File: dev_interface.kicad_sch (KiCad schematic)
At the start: 17 parts, among them U10 ADS1014IDGS, U11 ADS1014IDGS, U4 ISO164xB, U5 DACx53401, U6 DACx53401, U8 LM2904

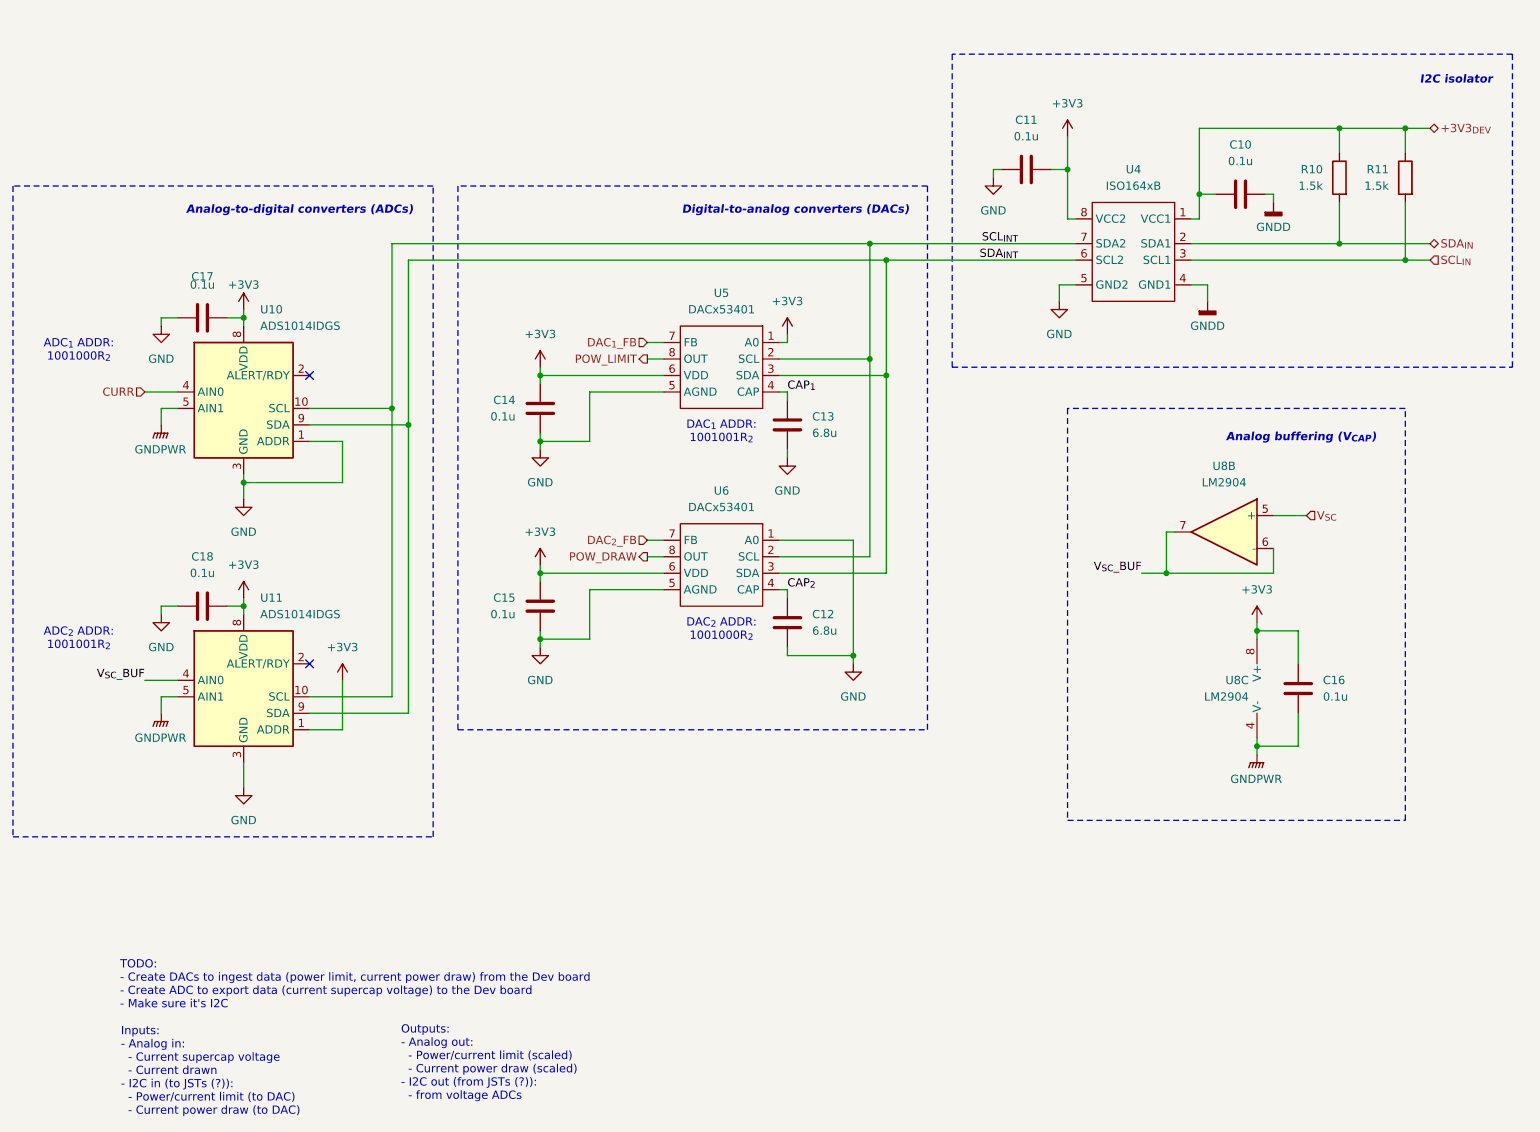
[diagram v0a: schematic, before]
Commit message: last formatting change I promise
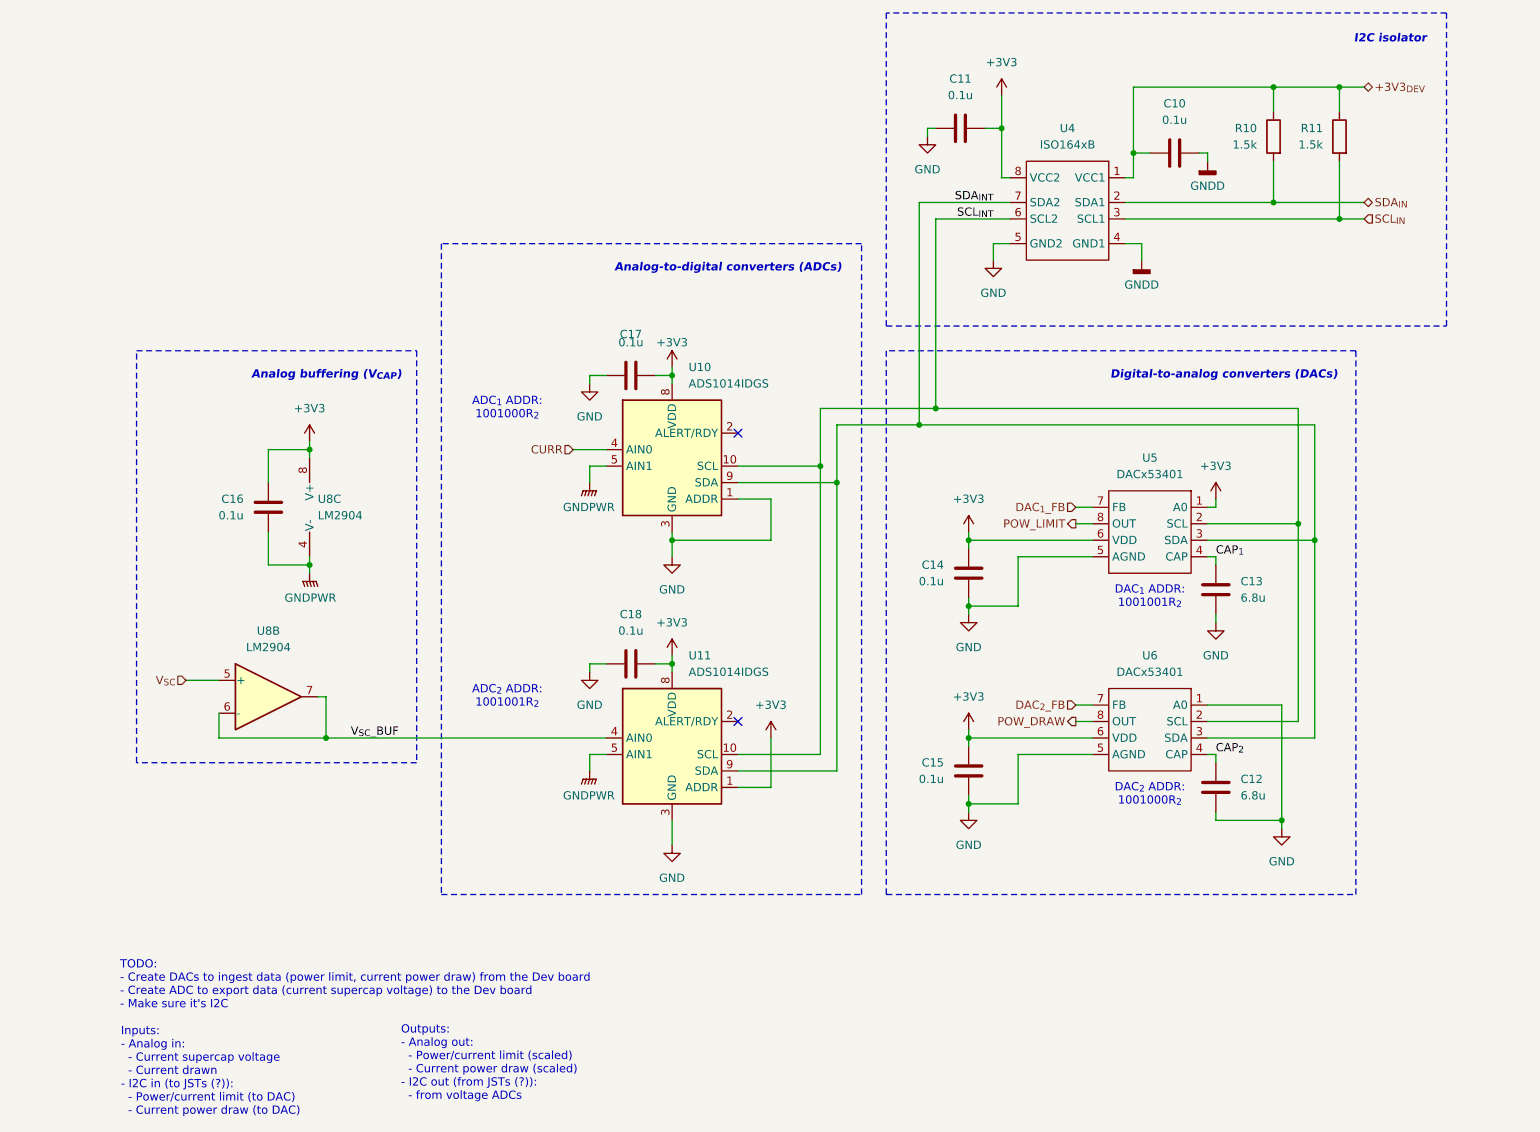
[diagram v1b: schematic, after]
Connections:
- net SCL_{INT}: now also U4.6 (SCL2); no longer U4.7 (SDA2)
- net SDA_{INT}: now also U4.7 (SDA2); no longer U4.6 (SCL2)
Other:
- moved on the sheet: C10, C11, C12, C13, C14, C15, C16, C17, C18, R10, R11, U10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
